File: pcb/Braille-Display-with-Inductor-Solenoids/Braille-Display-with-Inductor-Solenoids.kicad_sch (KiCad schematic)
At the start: 13 parts, among them J1 Screw_Terminal_01x02, J2 Screw_Terminal_01x02, J3 Screw_Terminal_01x02, SW1 SW_Push, SW2 SW_Push, U1 RP2040-Zero

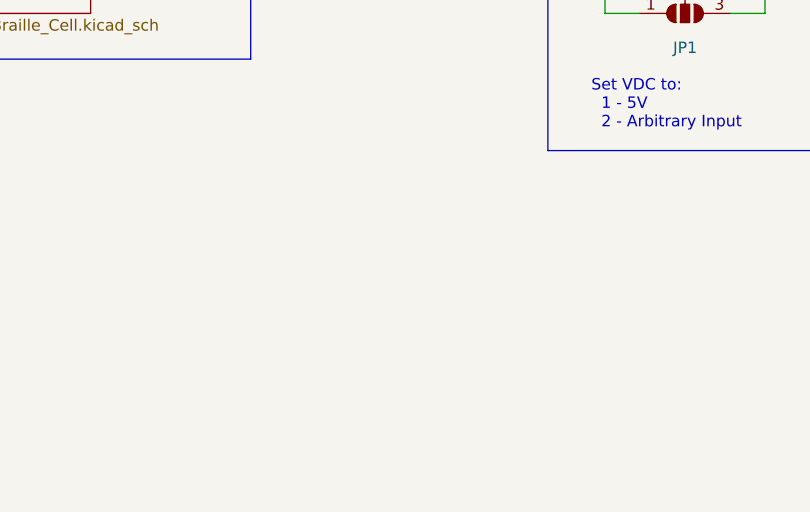
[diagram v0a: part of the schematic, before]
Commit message: Finish up board
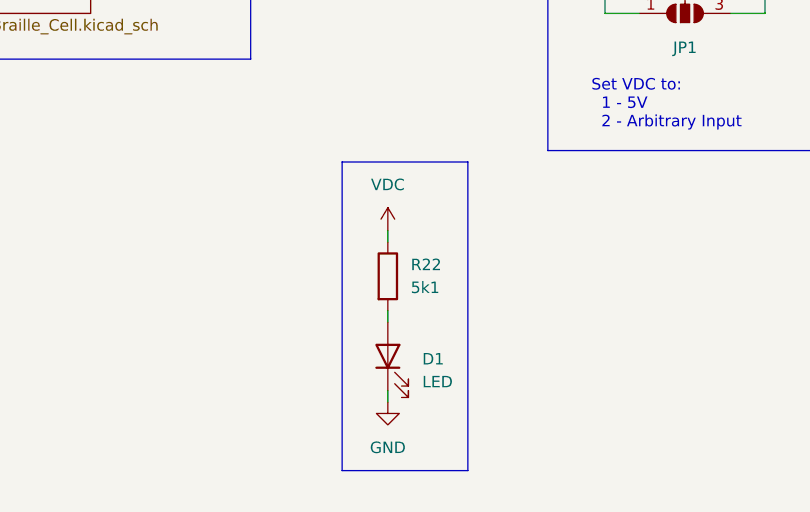
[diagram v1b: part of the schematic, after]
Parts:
- added D1: LED, LED_SMD:LED_1206_3216Metric_Pad1.42x1.75mm_HandSolder, symbol Device:LED
- added R22: 5k1, Resistor_SMD:R_1206_3216Metric_Pad1.30x1.75mm_HandSolder, symbol Device:R
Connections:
- net GND: now also D1.1 (K)
- net VDC: now also R22.1
- new net: D1.2 (A), R22.2
